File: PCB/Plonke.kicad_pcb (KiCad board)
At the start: 2 copper layers, 232 x 103.5 mm, 124 parts, among them J1 USB_C_Receptacle_USB2.0_16P, J2 AVR-ISP-6, SW1 SW_Push, SW10 SW_Push, SW11 SW_Push, SW12 SW_Push, SW13 SW_Push, SW14 SW_Push, SW15 SW_Push, SW16 SW_Push, SW17 SW_Push, SW18 SW_Push, SW19 SW_Push, SW2 SW_Push, SW20 SW_Push, SW21 SW_Push, SW22 SW_Push, SW23 SW_Push, SW24 SW_Push, SW25 SW_Push, SW26 SW_Push, SW27 SW_Push, SW28 SW_Push, SW29 SW_Push, SW3 SW_Push, SW30 SW_Push, SW31 SW_Push, SW32 SW_Push, SW33 SW_Push, SW34 SW_Push, SW35 SW_Push, SW36 SW_Push, SW37 SW_Push, SW38 SW_Push, SW39 SW_Push, SW4 SW_Push, SW40 SW_Push, SW41 SW_Push, SW42 SW_Push, SW43 SW_Push, SW44 SW_Push, SW45 SW_Push, SW46 SW_Push, SW47 SW_Push, SW5 SW_Push, SW6 SW_Push, SW7 SW_Push, SW8 SW_Push, SW9 SW_Push, U2 USB6B1, U3 ATmega328-P, Y1 Crystal_GND24_Small

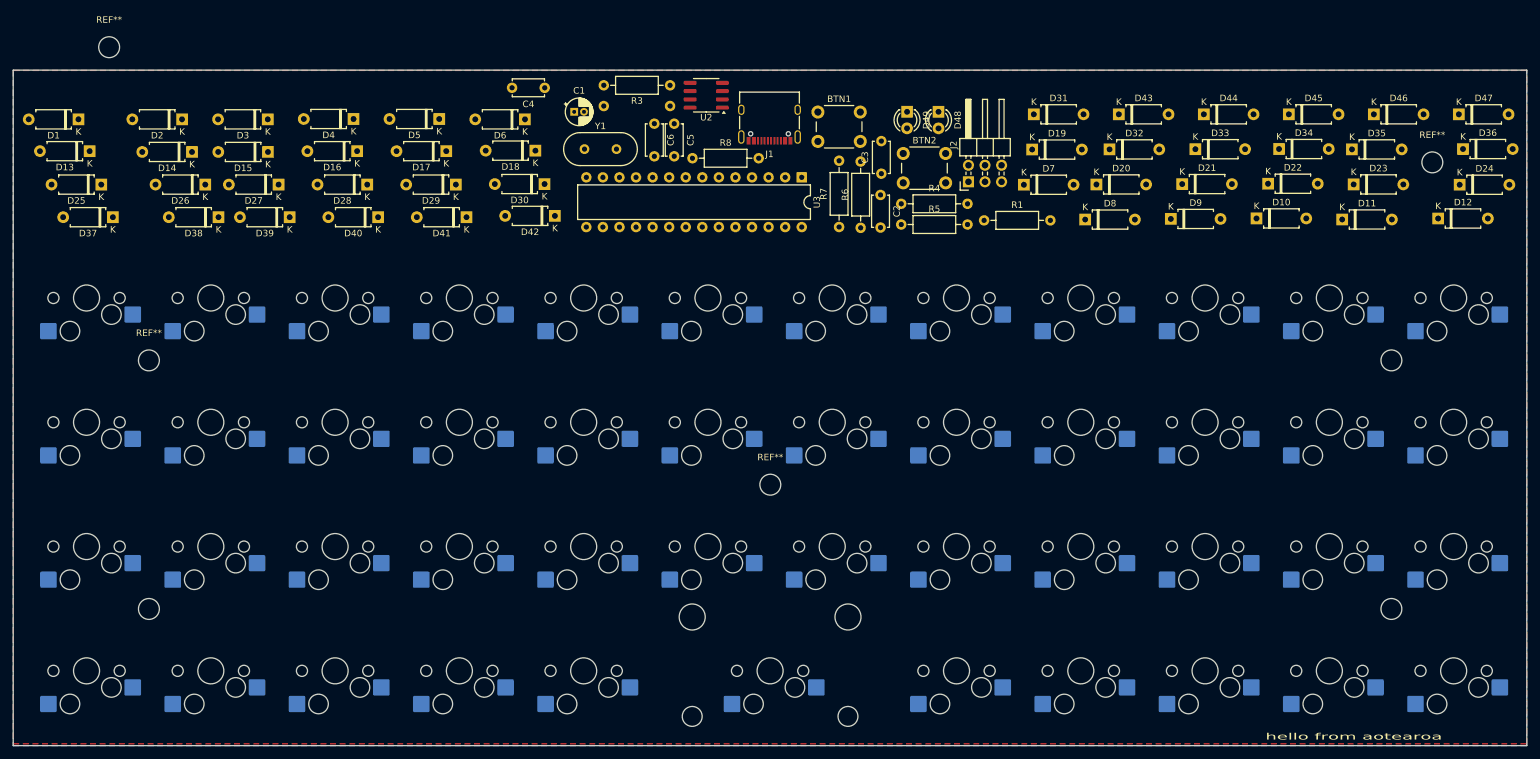
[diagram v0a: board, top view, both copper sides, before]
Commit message: i did this
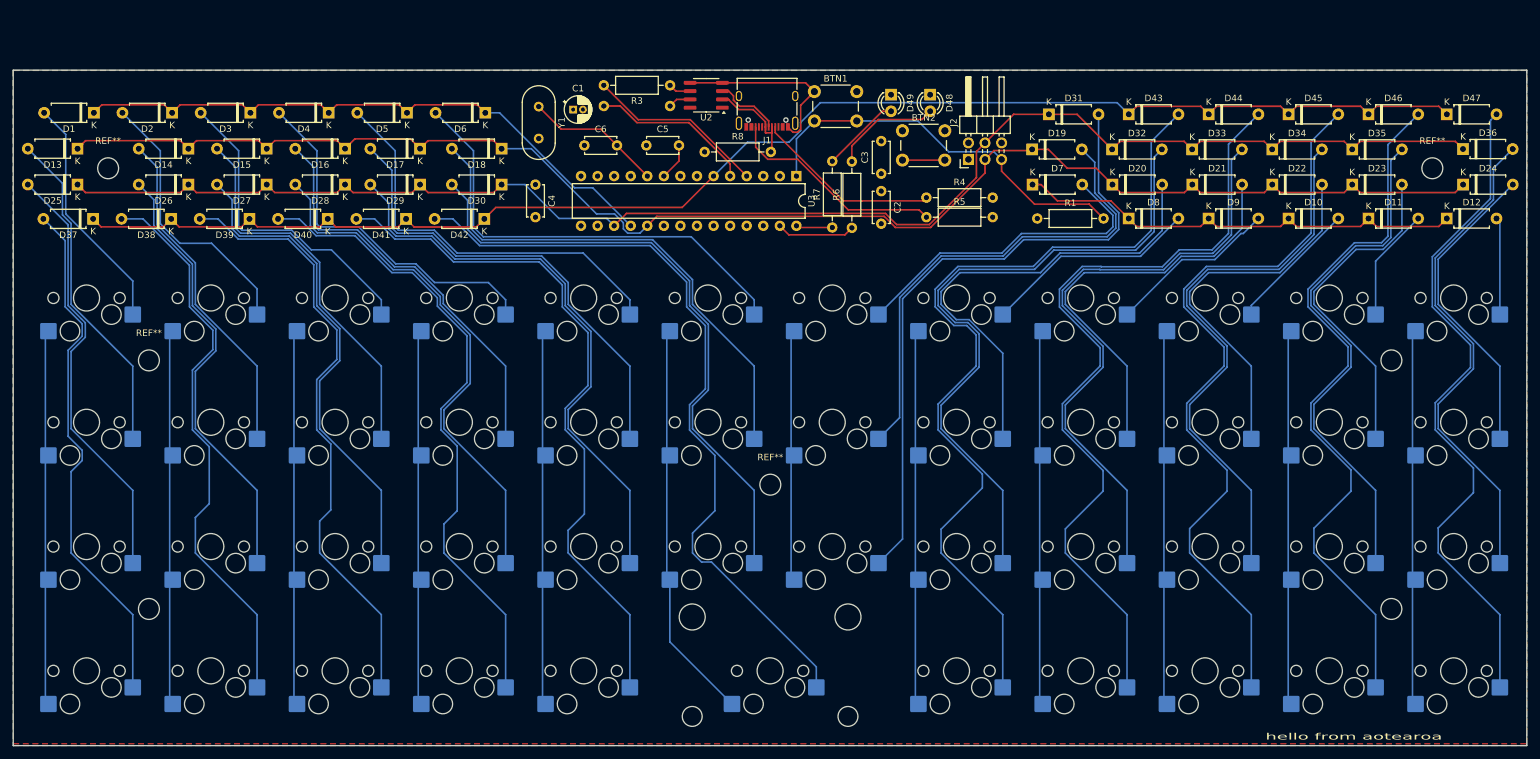
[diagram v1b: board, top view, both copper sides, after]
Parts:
- moved REF** 18.6 mm to (48.5, 58.5)
- moved C4 14.9 mm to (114.0, 61.0), turned to -90 degrees
- moved C6 11.2 mm to (121.5, 55.0), turned to 0 degrees
- moved D42 10.8 mm to (106.2, 66.3)
- moved Y1 9.57 mm to (114.5, 49.0), turned to -90 degrees
- moved D41 9.27 mm to (94.2, 66.3)
- moved R1 8.16 mm to (191.0, 66.2)
- moved D40 7.72 mm to (82.2, 66.3)
- moved D38 7.26 mm to (58.2, 66.3)
- moved D8 6.67 mm to (205.0, 66.2)
- moved D30 6.58 mm to (108.9, 61.0)
- moved D39 6.17 mm to (70.2, 66.3)
- moved D6 6.16 mm to (106.4, 50.0)
- moved D9 5.79 mm to (217.2, 66.2)
- moved D29 5.49 mm to (96.4, 61.0)
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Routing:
- net R2: track 0.00 -> 237.8 mm
- net MOSI: track 0.00 -> 237.2 mm
- net R4: track 0.00 -> 225.5 mm
- net MISO: track 0.00 -> 164.3 mm
- net Net-(D43-A): track 0.00 -> 132.9 mm
- net Net-(D44-A): track 0.00 -> 124.6 mm
- net Net-(D42-A): track 0.00 -> 118.7 mm
- net Net-(D45-A): track 0.00 -> 117.9 mm
- net Net-(D46-A): track 0.00 -> 111.0 mm
- net Net-(D41-A): track 0.00 -> 106.7 mm
- net Net-(D47-A): track 0.00 -> 105.2 mm
- net Net-(D32-A): track 0.00 -> 101.8 mm
- net Net-(D31-A): track 0.00 -> 98.5 mm
- net Net-(D40-A): track 0.00 -> 98.5 mm
- net Net-(D30-A): track 0.00 -> 94.5 mm
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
